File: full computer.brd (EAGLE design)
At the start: 153.9 x 87 mm, 71 parts, among them IC2 74HC541N, IC3 74HC573N, IC4 74HC04N, Q1 IRF9530

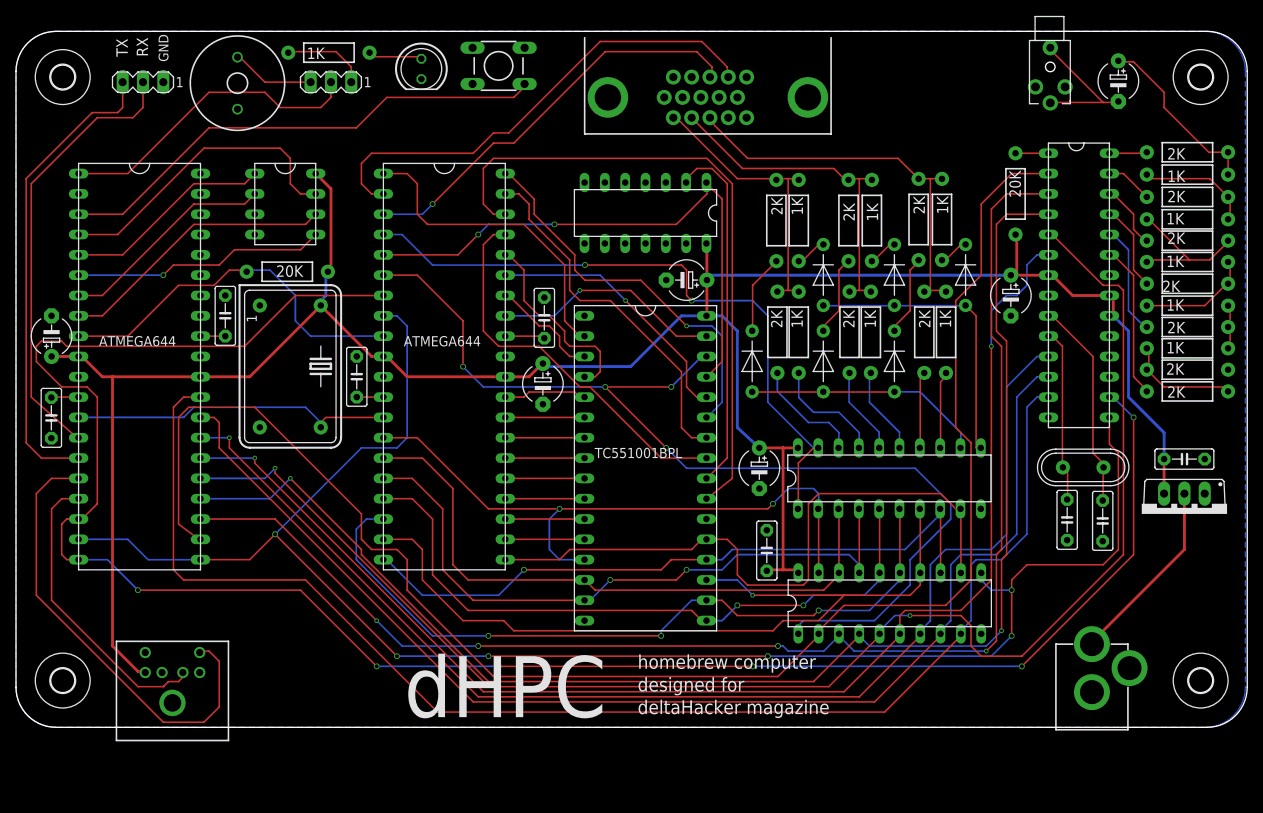
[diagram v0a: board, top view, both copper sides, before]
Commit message: board completely redesigned!
Signed-off-by: Panagiotis Varelas <varelaspanos@gmail.com>
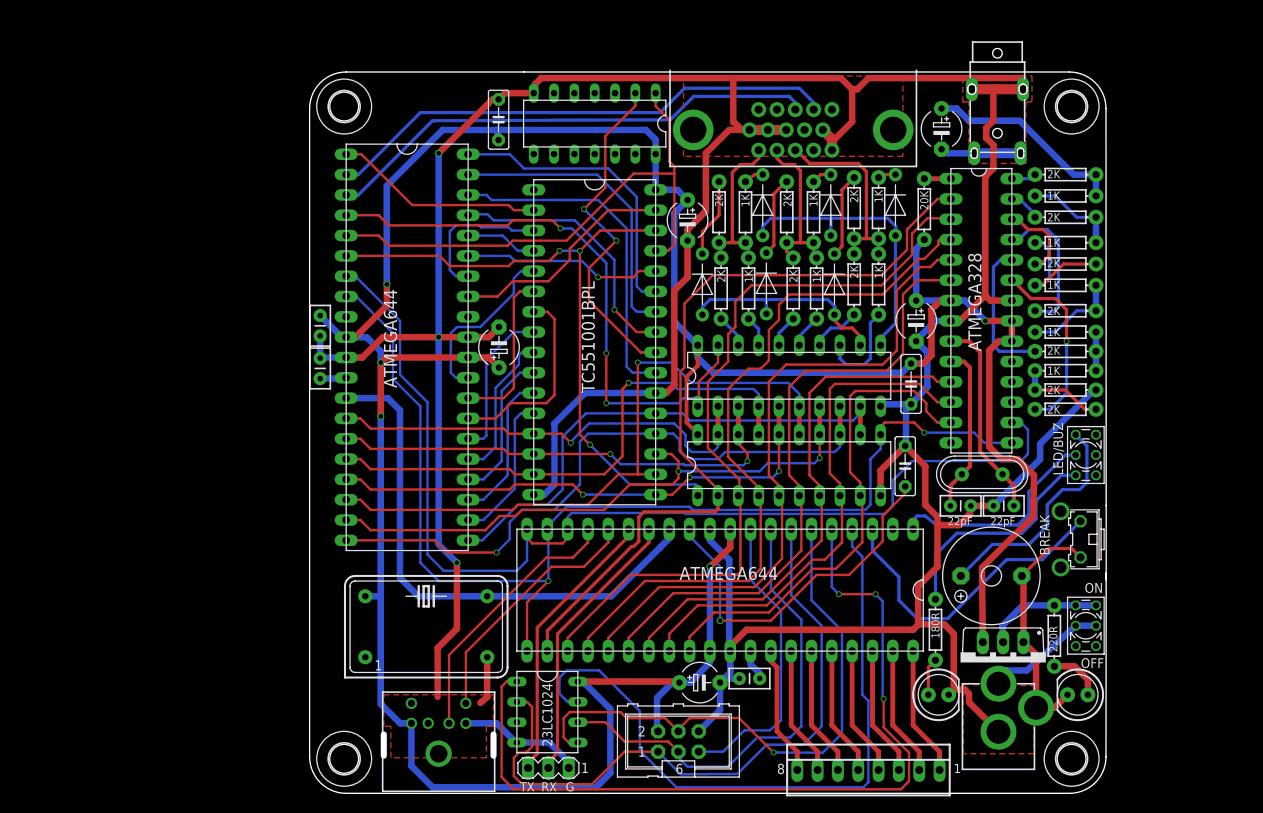
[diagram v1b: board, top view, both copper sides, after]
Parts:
- removed BREAK: TACTILE-SWITCH-PTH, GeekAmmo:TAC-SWITCH-PTH
- removed BUZZER: BUZZERNS, SparkFun-Electromechanical:BUZZER-12MM-NS
- removed C4: 6.8uF, rcl:E5-5
- removed C7: 100nF, capacitor-wima:C5B2.5
- removed JMP: (no value), con-lstb:MA03-1
- removed JP1: AUDIO, SparkFun-Connectors:STEREOJACK2.5MM_STEREOJACK2.5MM
- added C6: 100nF, SparkFun-Capacitors:CAP-PTH-SMALLEZ
- added D1: (no value), SparkFun-LED:LED5MM
- added GPIO: 22-23-2081, con-molex:22-23-2081
- added ISP: (no value), con-ml:ML6
- added S1, S3: 9450-2, switch-misc:9450-2
- added S2: (no value), switch-omron:B3F-31XX
- added SG1: F/TMB, buzzer:F/TMB
- added X1: 1503_08, con-lumberg:1503_08
- C14, C15: device capacitor-wima:C5B2.5 -> SparkFun-Passives:CAP-PTH-SMALLEZ
- C2, C5: device capacitor-wima:C5B2.5 -> SparkFun-Capacitors:CAP-PTH-SMALLEZ
- H1, H2, H4, H5: device holes:3,0 -> holes:3,6
- JP2: value POWER 5V -> 5V
- LED1: device led:LED5MM -> SparkFun-LED:LED5MM
- U$11, U$12, U$13, U$14, U$15, U$16, U$26, U$27, U$28, U$29, U$30, U$31, U$32, U$33, U$34, U$35, U$36, U$37, U$38, U$4, U$5, U$6, U$7, U$8, U$9: device SparkFun-Resistors:AXIAL-0.4 -> SparkFun-Resistors:AXIAL-0.3EZ
- U$23: value 20K -> 220R; device SparkFun-Resistors:AXIAL-0.4 -> SparkFun-Resistors:AXIAL-0.3EZ
- U$24: value 1K -> 180R; device SparkFun-Resistors:AXIAL-0.4 -> SparkFun-Resistors:AXIAL-0.3EZ
- moved C10 106.9 mm to (113.7, 51.1), turned to 90 degrees
- moved U$23 106.1 mm to (132.3, 29.8), turned to 90 degrees
- moved U$24 104.7 mm to (117.5, 30.6), turned to 90 degrees
- moved LED1 101.5 mm to (117.9, 22.5), turned to 0 degrees
- moved JMP1 99.6 mm to (69.1, 13.3)
- moved C1 95.6 mm to (62.9, 94.4), turned to 90 degrees
- moved C12 91.9 mm to (88.0, 24.0), turned to 0 degrees
- moved C2 80.7 mm to (95.5, 24.5), turned to 180 degrees
- moved U$1 79.4 mm to (91.8, 35.6), turned to 270 degrees
- moved U$10 71.5 mm to (69.0, 20.3)
- moved QG1 36.7 mm to (53.8, 31.0), turned to 0 degrees
- moved H5 36.5 mm to (43.6, 14.5)
- moved H1 35.4 mm to (43.6, 96.0)
- moved U$39 33.9 mm to (55.4, 10.4)
- moved Q1 29.3 mm to (125.9, 26.5)
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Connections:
- removed net N$46: C7.1, U$2.AREF
- new net N$54: GPIO.2, U$1.PA6
- new net N$55: GPIO.3, U$1.PA5
- new net N$56: GPIO.4, U$1.PA4
- new net N$57: GPIO.5, U$1.PA3
- new net N$58: GPIO.6, U$1.PA2
- new net N$59: GPIO.7, U$1.PA1
- new net N$60: GPIO.8, U$1.PA0
- new net N$61: ISP.5, U$1.~RESET
- new net N$64: Q1.D, S3.1, S3.4, U$23.P$2
- new net N$69: D1.A, U$23.P$1
- net AUDIO-OUT: now also X1.1, X1.3; no longer JP1.SHIELD, JP1.TIP
- net GND: now also C6.2, D1.K, ISP.6, S2.1, SG1.-, X1.2@1, X1.2@2; no longer BREAK.2, BUZZER.-, C4.-, C7.2, JP1.RING1
- net N$17: now also S3.2, S3.5; no longer Q1.D
- net N$18: now also S1.1, SG1.+; no longer BUZZER.+, JMP.3
- net N$19: now also S1.3; no longer JMP.1
- net N$21: now also S1.2; no longer JMP.2
- net N$4: now also GPIO.1, U$1.PA7; no longer U$1.~RESET, U$2.~RESET, U$23.P$1
- net N$48: now also ISP.3
- net N$49: now also S2.2; no longer BREAK.4
- net N$50: now also ISP.1
- net N$51: now also ISP.4
- net VCC: now also C6.1, ISP.2; no longer C4.+, U$23.P$2
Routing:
- net GND: track 0.00 -> 521.5 mm, vias 0 -> 3
- net TO_CPU: track 247.3 -> 135.0 mm, vias 6 -> 0
- net CPUDATA7: track 171.2 -> 62.3 mm
- net CPUDATA3: track 185.8 -> 83.8 mm, vias 2 -> 0
- net CPUDATA0: track 198.8 -> 100.2 mm
- net CPUDATA6: track 154.4 -> 64.6 mm
- net VCC: track 290.9 -> 378.7 mm, vias 0 -> 5
- net CPUDATA5: track 153.0 -> 66.1 mm, vias 1 -> 0
- net CPUDATA4: track 163.8 -> 79.0 mm, vias 2 -> 0
- net CPUDATA2: track 174.9 -> 90.2 mm, vias 2 -> 0
- net N$52: track 26.2 -> 103.6 mm, vias 0 -> 3
- net CPUDATA1: track 171.4 -> 96.5 mm, vias 4 -> 0
- net FROM_CPU: track 209.4 -> 141.5 mm, vias 6 -> 2
- net N$50: track 27.3 -> 82.7 mm
- net N$8: track 130.1 -> 82.6 mm, vias 4 -> 3
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- added copper zone on layer 1, net GND
- removed copper zone on layer 16, net GND
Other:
- board size 153.9 x 87 mm -> 99.6 x 90.2 mm
- board text added: "1"
- board text added: "100nF"
- board text added: "2"
- board text added: "20MHz"
- board text added: "22pF"
- board text added: "23LC1024"
- board text added: "6.8uF"
- board text added: "8"
- board text added: "APU"
- board text added: "AUDIO"
- board text added: "BREAK"
- board text added: "BUZZER"
- board text added: "CLOCK"
- board text added: "CPU"
- board text added: "DAC"
- board text added: "G"
- board text added: "GPIO"
- board text added: "GPU"
- board text added: "KEYBOARD"
- board text added: "LED/BUZ"
- board text added: "MONITOR"
- board text added: "OFF"
- board text added: "ON"
- board text added: "POWER"
- board text added: "SPK"
- board text added: "SRAM"
- board text added: "SYSTEM"
- board text added: "VIDEO DAC"
- board text added: "VRAM"
- board text added: "by spir@l evolut10n"
- board text removed: "DEC 2015"
- board text removed: "GND"
- board text removed: "by pvar aka spir@l evolut10n"
- board text removed: "homebrew computer designed for deltaHacker magazine"
